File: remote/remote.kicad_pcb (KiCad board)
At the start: 2 copper layers, 38 x 88 mm, 57 parts, among them J1 Conn_01x04, J2 Conn_01x05, Q1 AO3401A, Q2 AO3401A, Q3 AO3401A, Q4 AO3401A, SW1 SW_Push, SW2 SW_Push, SW3 SW_Push, SW4 SW_Push, U1 STM32F030F4Px, U2 RFM69CW-915MHZ

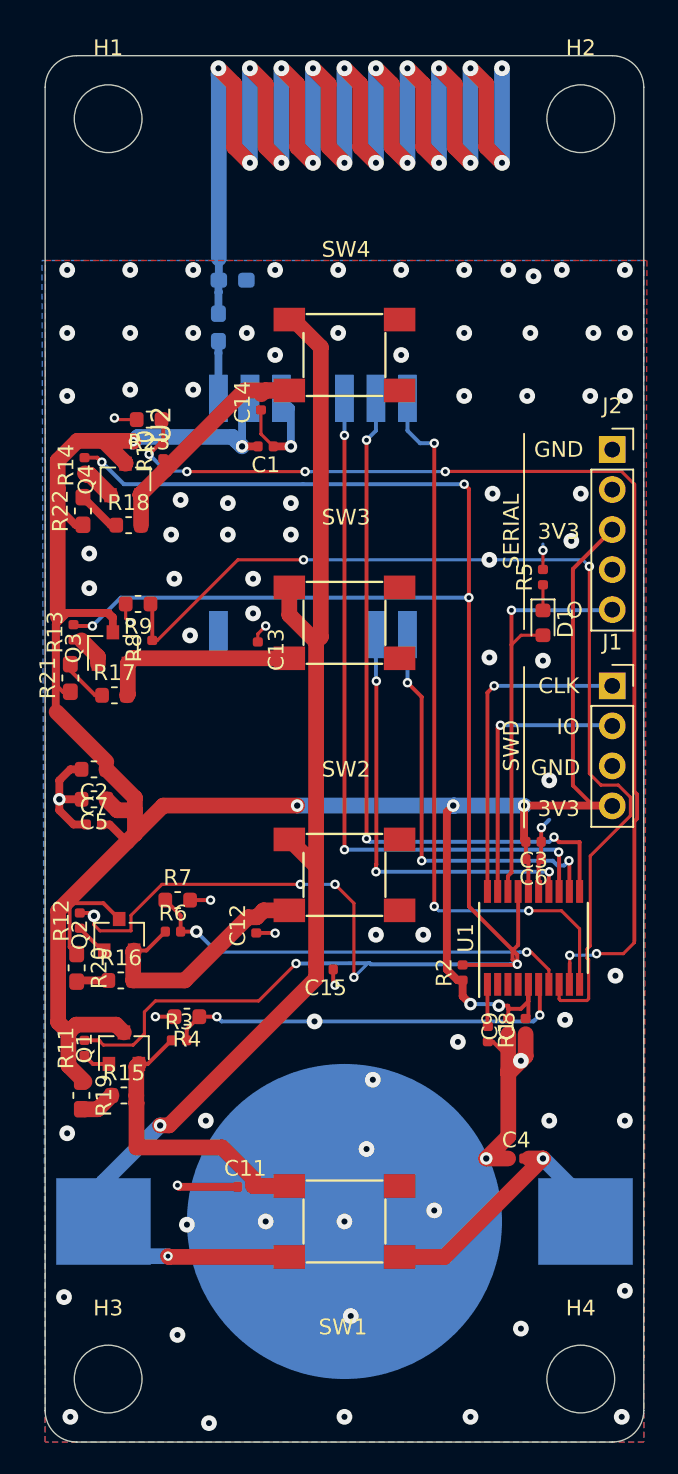
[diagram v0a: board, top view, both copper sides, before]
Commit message: Update layout for v1.1
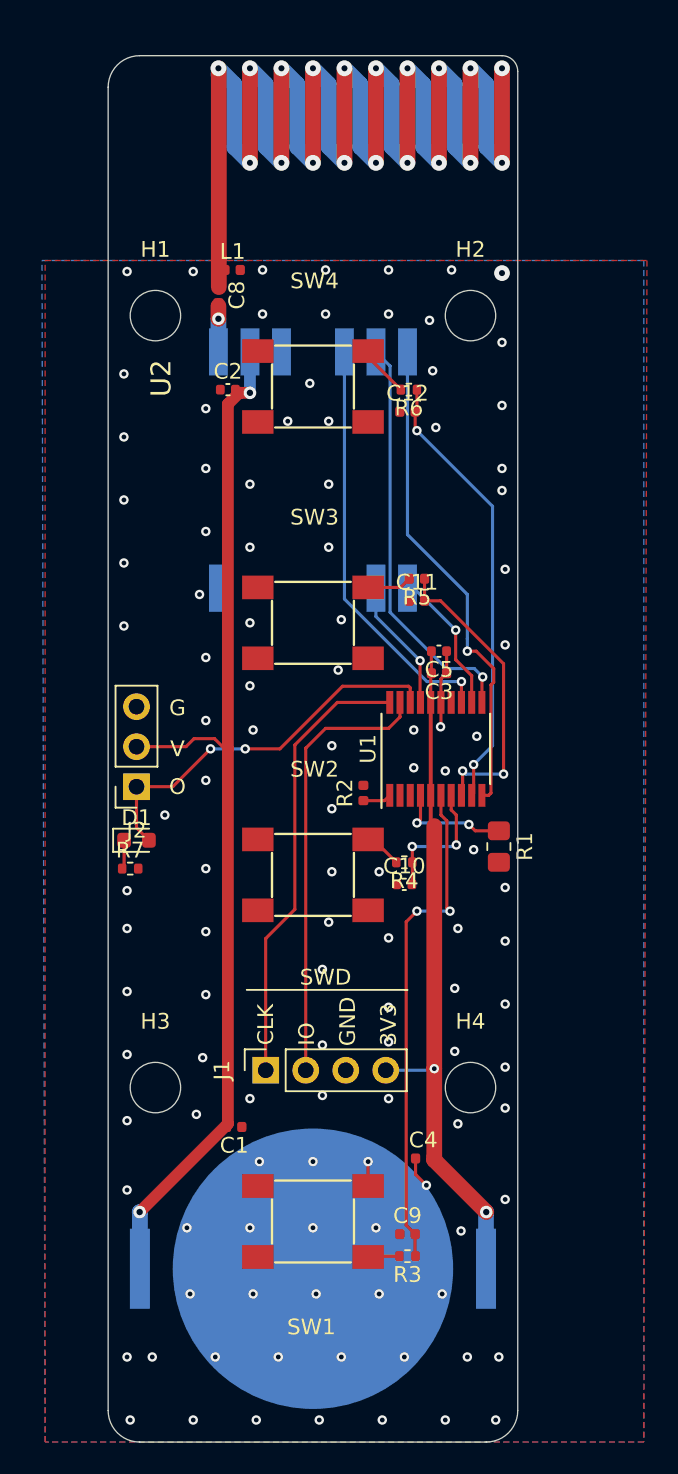
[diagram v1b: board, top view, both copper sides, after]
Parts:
- removed C13, C14: 1uF, Capacitor_SMD:C_0402_1005Metric
- removed C15, C6, C7: .1uF, Capacitor_SMD:C_0402_1005Metric
- removed Q1, Q2, Q3, Q4: AO3401A, Package_TO_SOT_SMD:SOT-23
- removed R10, R8: 47k, Resistor_SMD:R_0402_1005Metric
- removed R11, R12, R13, R14: 1k, Resistor_SMD:R_0402_1005Metric
- removed R15, R16, R17, R18: 5.1, Resistor_SMD:R_0603_1608Metric
- removed R19, R20, R21, R22: 0, Resistor_SMD:R_0603_1608Metric_Pad1.05x0.95mm_HandSolder
- removed R23, R9: 680k, Resistor_SMD:R_0603_1608Metric
- BT1: footprint Battery:BatteryHolder_Keystone_3008_1x2450 -> Battery:BatteryHolder_Keystone_3034_1x20mm
- C1: value .1uF -> 1uF
- C10: value 1pF -> 1uF; footprint Capacitor_SMD:C_0603_1608Metric_Pad1.05x0.95mm_HandSolder -> Capacitor_SMD:C_0402_1005Metric; moved to F.Cu
- C2, C5: value 22uF -> .1uF; footprint Capacitor_SMD:C_0603_1608Metric -> Capacitor_SMD:C_0402_1005Metric
- C8: value .1uF -> 1pF
- H1, H2, H3, H4: footprint MountingHole:MountingHole_4.3mm_M4_ISO14580 -> MountingHole:MountingHole_3.2mm_M3
- J2: value Conn_01x05 -> Conn_01x03; footprint Connector_PinSocket_2.54mm:PinSocket_1x05_P2.54mm_Vertical -> Connector_PinSocket_2.54mm:PinSocket_1x03_P2.54mm_Vertical
- L1: footprint Inductor_SMD:L_0603_1608Metric_Pad1.05x0.95mm_HandSolder -> Inductor_SMD:L_0402_1005Metric; moved to F.Cu
- R1: value 15k -> DNP; footprint Resistor_SMD:R_0402_1005Metric -> Resistor_SMD:R_0805_2012Metric_Pad1.20x1.40mm_HandSolder
- R3, R6: value 47k -> 1k
- R4, R7: value 680k -> 1k; footprint Resistor_SMD:R_0603_1608Metric -> Resistor_SMD:R_0402_1005Metric
- moved C8 50.3 mm to (41.0, 45.2), turned to 270 degrees
- moved C1 43.2 mm to (42.0, 98.0)
- moved C11 38.8 mm to (53.6, 64.6)
- moved R6 37.5 mm to (53.1, 51.2), turned to 180 degrees
- moved C10 37.3 mm to (52.8, 82.6), turned to 0 degrees
- moved J2 37.0 mm to (35.8, 76.4), turned to 180 degrees
- moved C12 34.0 mm to (53.0, 52.6), turned to 0 degrees
- moved J1 32.9 mm to (44.0, 94.4), turned to 90 degrees
- moved D1 29.3 mm to (35.8, 79.8), turned to 0 degrees
- moved C2 25.6 mm to (41.6, 51.2), turned to 0 degrees
- moved C5 23.8 mm to (55.0, 67.8)
- moved R3 19.9 mm to (53.0, 106.2), turned to 180 degrees
- moved H4 19.8 mm to (57.0, 95.5)
- moved H3 18.7 mm to (37.0, 95.5)
- moved R4 16.9 mm to (52.8, 81.2)
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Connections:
- BT1 pad 1: +BATT -> VCC
- C10 pad 1: /ANTENNA -> GND
- C10 pad 2: Net-(C10-Pad2) -> /SW_2
- C11 pad 2: Net-(C11-Pad2) -> /SW_3
- C12 pad 2: Net-(C12-Pad2) -> /SW_4
- C2 pad 1: VCC -> GND
- C2 pad 2: GND -> VCC
- C4 pad 2: +BATT -> VCC
- C5 pad 1: VCC -> GND
- C5 pad 2: GND -> VCC
- C8 pad 1: GND -> /ANTENNA
- C8 pad 2: VCC -> Net-(C8-Pad2)
- C9 pad 2: VCC -> /SW_1
- J2 pad 1: GND -> /SERIAL_OUT
- J2 pad 2: (no net) -> VCC
- J2 pad 3: VCC -> GND
- R2 pad 1: VCC -> Net-(R2-Pad1)
- R2 pad 2: /SENSE_BYPASS -> GND
- R3 pad 1: Net-(C11-Pad2) -> /SW_1
- R3 pad 2: /SENSE_1 -> Net-(R3-Pad2)
- R4 pad 1: /SENSE_1 -> /SW_2
- R4 pad 2: GND -> Net-(R4-Pad2)
- R5 pad 1: Net-(D1-Pad1) -> /SW_3
- R5 pad 2: GND -> Net-(R5-Pad2)
- R6 pad 1: Net-(C12-Pad2) -> /SW_4
- R6 pad 2: /SENSE_2 -> Net-(R6-Pad2)
- R7 pad 1: /SENSE_2 -> Net-(D1-Pad1)
- SW1 pad 1: +BATT -> Net-(R3-Pad2)
- SW1 pad 2: Net-(C11-Pad2) -> GND
- SW2 pad 1: +BATT -> Net-(R4-Pad2)
- SW2 pad 2: Net-(C12-Pad2) -> GND
- SW3 pad 1: +BATT -> Net-(R5-Pad2)
- SW3 pad 2: Net-(C13-Pad2) -> GND
- SW4 pad 1: +BATT -> Net-(R6-Pad2)
- SW4 pad 2: Net-(C14-Pad2) -> GND
- U1 pad 1: Net-(R1-Pad1) -> Net-(R2-Pad1)
- U1 pad 14: /RADIO_DIO0 -> (no net)
- U1 pad 17: /SENSE_BYPASS -> /RADIO_DIO0
- U1 pad 4: (no net) -> Net-(R1-Pad1)
- U1 pad 6: /SENSE_1 -> /SW_1
- U1 pad 7: /SENSE_2 -> /SW_2
- U1 pad 8: /SENSE_3 -> /SW_3
- U1 pad 9: /SENSE_4 -> /SW_4
- U2 pad 1: Net-(C10-Pad2) -> Net-(C8-Pad2)
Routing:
- net /SENSE_BYPASS: track 148.1 -> 0.00 mm, vias 10 -> 0
- net +BATT: track 104.1 -> 0.00 mm, vias 3 -> 0
- net /SENSE_4: track 70.3 -> 0.00 mm, vias 6 -> 0
- net VCC: track 178.4 -> 111.6 mm, vias 7 -> 4
- net /SENSE_3: track 65.6 -> 0.00 mm, vias 3 -> 0
- net GND: track 64.2 -> 8.50 mm, vias 85 -> 112
- net /SW_1: track 0.00 -> 32.1 mm, vias 0 -> 2
- net /SW_4: track 0.00 -> 28.4 mm, vias 0 -> 2
- net /SENSE_2: track 27.9 -> 0.00 mm, vias 2 -> 0
- net /SENSE_1: track 25.7 -> 0.00 mm, vias 3 -> 0
- net /SW_3: track 0.00 -> 19.3 mm, vias 0 -> 2
- net /RADIO_SCK: track 45.2 -> 26.1 mm, vias 3 -> 1
- net Net-(C11-Pad2): track 19.1 -> 0.00 mm
- net /RADIO_DIO0: track 27.3 -> 8.42 mm, vias 3 -> 1
- net /RADIO_MOSI: track 44.8 -> 26.7 mm, vias 3 -> 1
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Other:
- board size 38 x 88 mm -> 26 x 88 mm
- board text added: "CR2032"
- board text added: "G"
- board text added: "V"
- board text added: "home remote v1.1"
- board text added: "v1.1"
- board text removed: "1x CR2450"
- board text removed: "OUT"
- board text removed: "SERIAL"
- board text removed: "home remote v1.0"
